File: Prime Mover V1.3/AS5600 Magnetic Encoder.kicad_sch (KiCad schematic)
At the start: 1 part, among them J1 Conn_01x08_Male

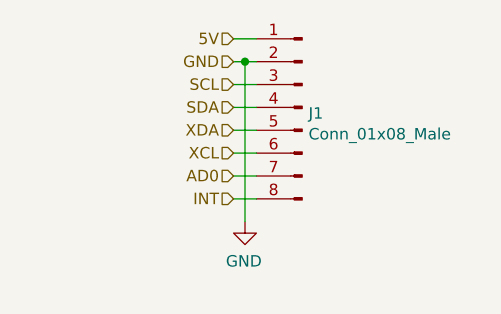
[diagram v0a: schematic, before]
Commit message: polished
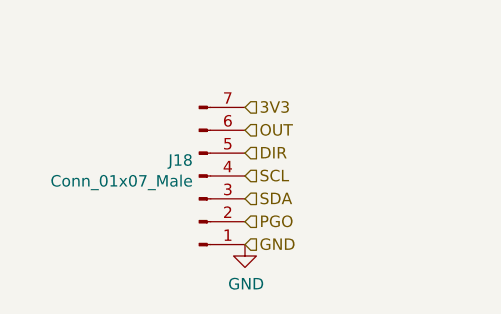
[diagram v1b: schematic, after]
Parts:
- removed J1: Conn_01x08_Male, RascalHat:MPU-6050-Module, symbol Connector:Conn_01x08_Male
- added J18: Conn_01x07_Male, Connector_JST:JST_PH_B7B-PH-K_1x07_P2.00mm_Vertical, symbol Connector:Conn_01x07_Male
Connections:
- net GND: now also J18.1 (Pin_1)
- net SCL: now also J18.4 (Pin_4)
- net SDA: now also J18.3 (Pin_3)
- new net 3V3: J18.7 (Pin_7)
- new net DIR: J18.5 (Pin_5)
- new net OUT: J18.6 (Pin_6)
- new net PGO: J18.2 (Pin_2)
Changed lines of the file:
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@@
 (kicad_sch (version 20211123) (generator eeschema)
   (paper "A4")
-  (junction (at 133.35 83.82) (diameter 0) (color 0 0 0 0)
+  (hierarchical_label "SDA" (shape input) (at 133.35 99.06 0)
+    (effects (font (size 1.27 1.27)) (justify left))
   )
-  (wire (pts (xy 132.08 99.06) (xy 134.62 99.06))
-    (stroke (width 0) (type default) (color 0 0 0 0))
+  (hierarchical_label "OUT" (shape input) (at 133.35 91.44 0)
+    (effects (font (size 1.27 1.27)) (justify left))
   )
-  (wire (pts (xy 132.08 86.36) (xy 134.62 86.36))
-    (stroke (width 0) (type default) (color 0 0 0 0))
+  (hierarchical_label "PGO" (shape input) (at 133.35 101.6 0)
+    (effects (font (size 1.27 1.27)) (justify left))
   )
-  (wire (pts (xy 132.08 83.82) (xy 133.35 83.82))
-    (stroke (width 0) (type default) (color 0 0 0 0))
+  (hierarchical_label "SCL" (shape input) (at 133.35 96.52 0)
+    (effects (font (size 1.27 1.27)) (justify left))
   )
-  (wire (pts (xy 132.08 96.52) (xy 134.62 96.52))
-    (stroke (width 0) (type default) (color 0 0 0 0))
+  (hierarchical_label "3V3" (shape input) (at 133.35 88.9 0)
+    (effects (font (size 1.27 1.27)) (justify left))
   )
-  (wire (pts (xy 132.08 91.44) (xy 134.62 91.44))
-    (stroke (width 0) (type default) (color 0 0 0 0))
+  (hierarchical_label "DIR" (shape input) (at 133.35 93.98 0)
+    (effects (font (size 1.27 1.27)) (justify left))
   )
-  (wire (pts (xy 132.08 81.28) (xy 134.62 81.28))
-    (stroke (width 0) (type default) (color 0 0 0 0))
+  (hierarchical_label "GND" (shape input) (at 133.35 104.14 0)
+    (effects (font (size 1.27 1.27)) (justify left))
   )
-  (wire (pts (xy 134.62 83.82) (xy 133.35 83.82))
-    (stroke (width 0) (type default) (color 0 0 0 0))
-  )
-  (wire (pts (xy 133.35 83.82) (xy 133.35 101.6))
-    (stroke (width 0) (type default) (color 0 0 0 0))
-  )
-  (wire (pts (xy 132.08 88.9) (xy 134.62 88.9))
-    (stroke (width 0) (type default) (color 0 0 0 0))
-  )
-  (wire (pts (xy 132.08 93.98) (xy 134.62 93.98))
-    (stroke (width 0) (type default) (color 0 0 0 0))
-  )
-  (hierarchical_label "AD0" (shape input) (at 132.08 96.52 180)
-    (effects (font (size 1.27 1.27)) (justify right))
-  )
-  (hierarchical_label "XDA" (shape input) (at 132.08 91.44 180)
-    (effects (font (size 1.27 1.27)) (justify right))
-  )
-  (hierarchical_label "SCL" (shape input) (at 132.08 86.36 180)
-    (effects (font (size 1.27 1.27)) (justify right))
-  )
-  (hierarchical_label "INT" (shape input) (at 132.08 99.06 180)
-    (effects (font (size 1.27 1.27)) (justify right))
-  )
-  (hierarchical_label "XCL" (shape input) (at 132.08 93.98 180)
-    (effects (font (size 1.27 1.27)) (justify right))
-  )
-  (hierarchical_label "5V" (shape input) (at 132.08 81.28 180)
-    (effects (font (size 1.27 1.27)) (justify right))
-  )
-  (hierarchical_label "GND" (shape input) (at 132.08 83.82 180)
-    (effects (font (size 1.27 1.27)) (justify right))
-  )
-  (hierarchical_label "SDA" (shape input) (at 132.08 88.9 180)
-    (effects (font (size 1.27 1.27)) (justify right))
-  )
-  (symbol (lib_id "power:GND") (at 133.35 101.6 0) (mirror y) (unit 1)
+  (symbol (lib_id "Connector:Conn_01x07_Male") (at 128.27 96.52 0) (mirror x) (unit 1)
     (in_bom yes) (on_board yes)
-    (property "Reference" "#PWR042" (id 0) (at 133.35 107.95 0)
+    (property "Reference" "J18" (id 0) (at 127.5588 94.7928 0)
+      (effects (font (size 1.27 1.27)) (justify right))
+    )
+    (property "Value" "Conn_01x07_Male" (id 1) (at 127.5588 97.1042 0)
+      (effects (font (size 1.27 1.27)) (justify right))
+    )
+    (property "Footprint" "Connector_JST:JST_PH_B7B-PH-K_1x07_P2.00mm_Vertical" (id 2) (at 128.27 96.52 0)
       (effects (font (size 1.27 1.27)) hide)
     )
-    (property "Value" "GND" (id 1) (at 133.223 105.9942 0))
-    (property "Footprint" "" (id 2) (at 133.35 101.6 0)
-      (effects (font (size 1.27 1.27)) hide)
-    )
-    (property "Datasheet" "" (id 3) (at 133.35 101.6 0)
-      (effects (font (size 1.27 1.27)) hide)
-    )
-    (pin "1")
-  )
-  (symbol (lib_id "Connector:Conn_01x08_Male") (at 139.7 88.9 0) (mirror y) (unit 1)
-    (in_bom yes) (on_board yes)
-    (property "Reference" "J1" (id 0) (at 140.4112 89.5604 0)
-      (effects (font (size 1.27 1.27)) (justify right))
-    )
-    (property "Value" "Conn_01x08_Male" (id 1) (at 140.4112 91.8718 0)
-      (effects (font (size 1.27 1.27)) (justify right))
-    )
-    (property "Footprint" "RascalHat:MPU-6050-Module" (id 2) (at 139.7 88.9 0)
-      (effects (font (size 1.27 1.27)) hide)
-    )
-    (property "Datasheet" "~" (id 3) (at 139.7 88.9 0)
+    (property "Datasheet" "~" (id 3) (at 128.27 96.52 0)
       (effects (font (size 1.27 1.27)) hide)
     )
@@
     (pin "6")
     (pin "7")
-    (pin "8")
+  )
+  (symbol (lib_id "power:GND") (at 133.35 104.14 0) (unit 1)
+    (in_bom yes) (on_board yes)
+    (property "Reference" "#PWR098" (id 0) (at 133.35 110.49 0)
+      (effects (font (size 1.27 1.27)) hide)
+    )
+    (property "Value" "GND" (id 1) (at 133.477 108.5342 0))
+    (property "Footprint" "" (id 2) (at 133.35 104.14 0)
+      (effects (font (size 1.27 1.27)) hide)
+    )
+    (property "Datasheet" "" (id 3) (at 133.35 104.14 0)
+      (effects (font (size 1.27 1.27)) hide)
+    )
+    (pin "1")
   )
 )
